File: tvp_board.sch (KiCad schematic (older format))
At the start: 60 parts, among them U1 TVP7002PZP, U4 SN74LVC2G17, U5 AP7361C, U6 TLV70033, U7 NCP703SN19T1G, U9 TLV70019, Y1 ACHL-27MHZ-EK

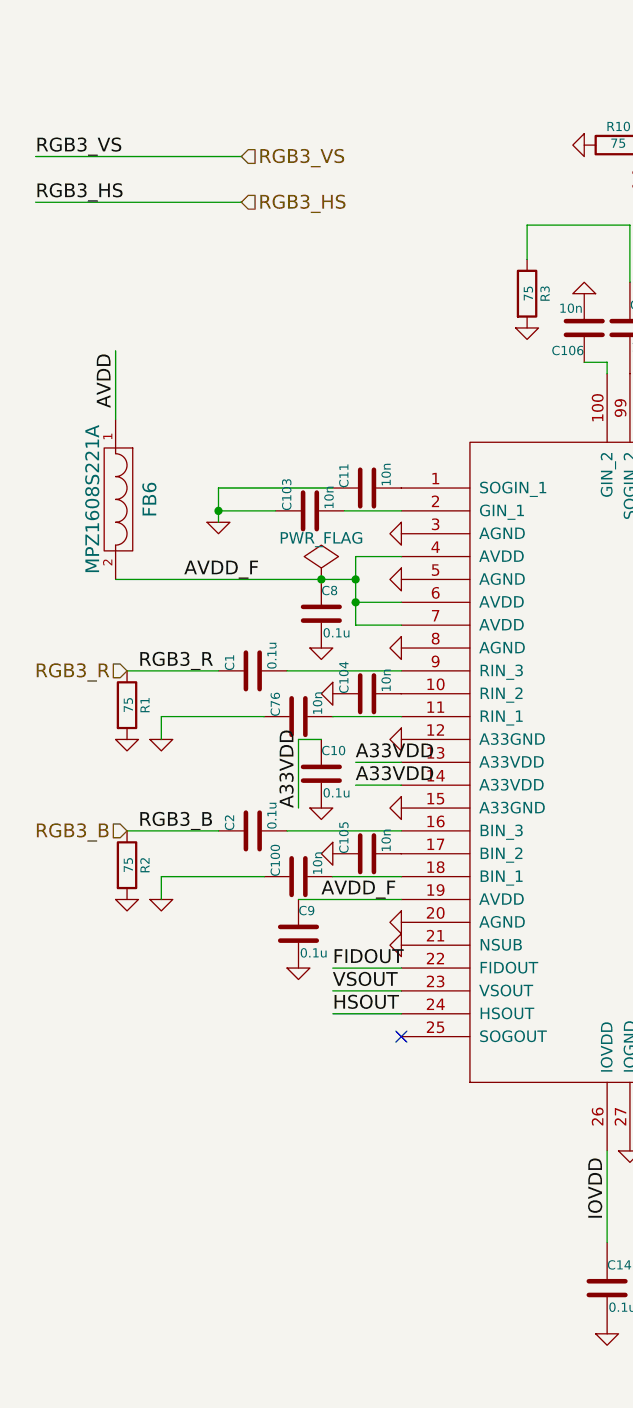
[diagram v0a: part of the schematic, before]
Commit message: update PCB 2
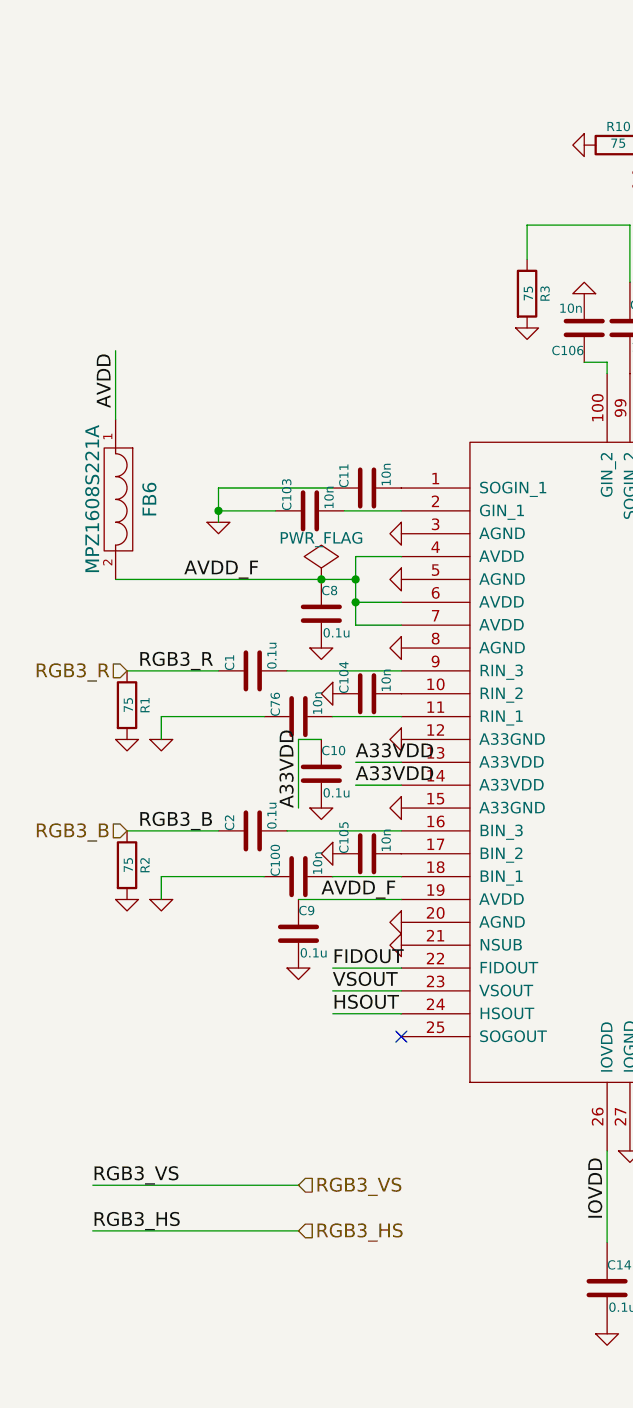
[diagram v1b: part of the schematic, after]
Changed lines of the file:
@@
 Text Label 10950 6550 0    60   ~ 0
 DVDD
-Text Label 2100 1350 0    60   ~ 0
+Text Label 2350 5850 0    60   ~ 0
 RGB3_HS
-Text Label 2100 1150 0    60   ~ 0
+Text Label 2350 5650 0    60   ~ 0
 RGB3_VS
 $Comp
@@
 	7450 6700 7550 6700
 Connection ~ 7450 6950
-Text HLabel 3000 1150 2    60   Input ~ 0
+Text HLabel 3250 5650 2    60   Input ~ 0
 RGB3_VS
-Text HLabel 3000 1350 2    60   Input ~ 0
+Text HLabel 3250 5850 2    60   Input ~ 0
 RGB3_HS
 Wire Wire Line
-	2100 1150 3000 1150
-Wire Wire Line
-	2100 1350 3000 1350
+	2350 5650 3250 5650
+Wire Wire Line
+	2350 5850 3250 5850
 Text HLabel 4800 800  2    60   Input ~ 0
 RGB3_G

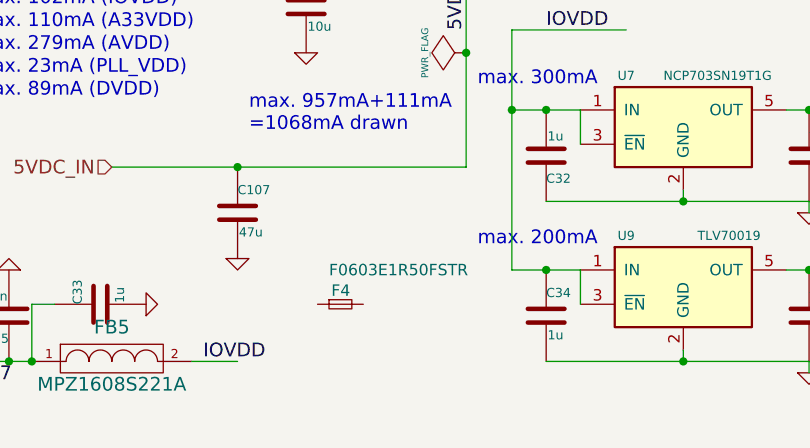
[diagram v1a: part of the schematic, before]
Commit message: update3
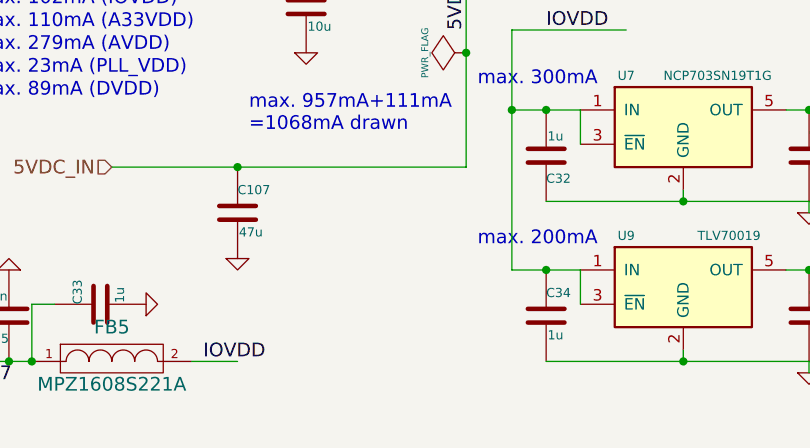
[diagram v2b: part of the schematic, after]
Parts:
- removed F4: F0603E1R50FSTR, Inductor_SMD:L_0603_1608Metric_Pad1.05x0.95mm_HandSolder, symbol ossc_board-rescue:F_Small
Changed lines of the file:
@@
-$EndComp
-$Comp
-L ossc_board-rescue:F_Small F4
-U 1 1 55ECFDAC
-P 8800 6700
-F 0 "F4" H 8760 6760 50  0000 L CNN
-F 1 "F0603E1R50FSTR" H 8750 6850 50  0000 L CNN
-F 2 "Inductor_SMD:L_0603_1608Metric_Pad1.05x0.95mm_HandSolder" H 8800 6700 60  0001 C CNN
-F 3 "" H 8800 6700 60  0000 C CNN
-	1    8800 6700
-	1    0    0    -1
 $EndComp
 $Comp

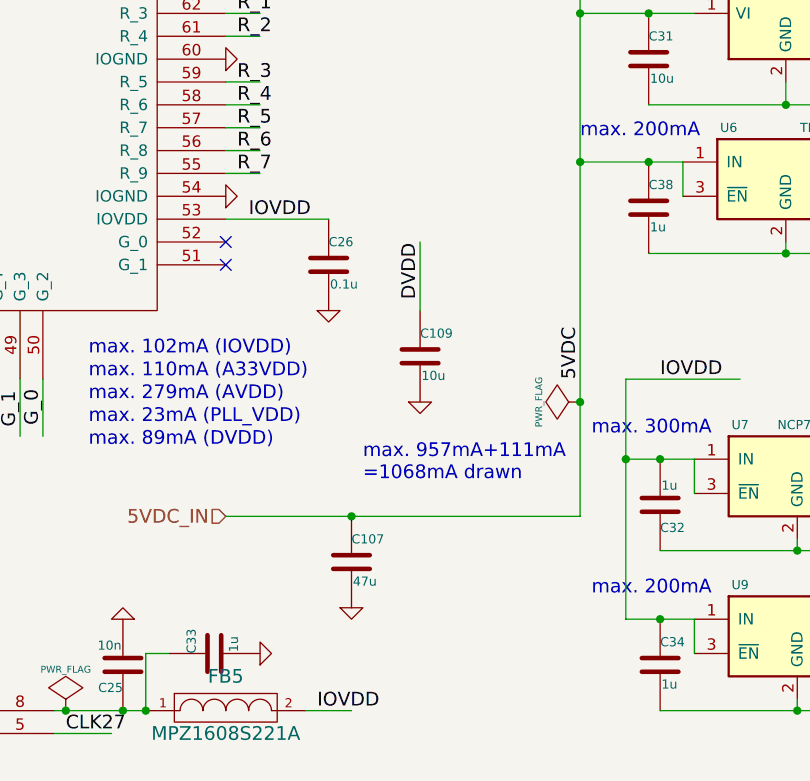
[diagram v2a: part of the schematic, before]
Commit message: minor update
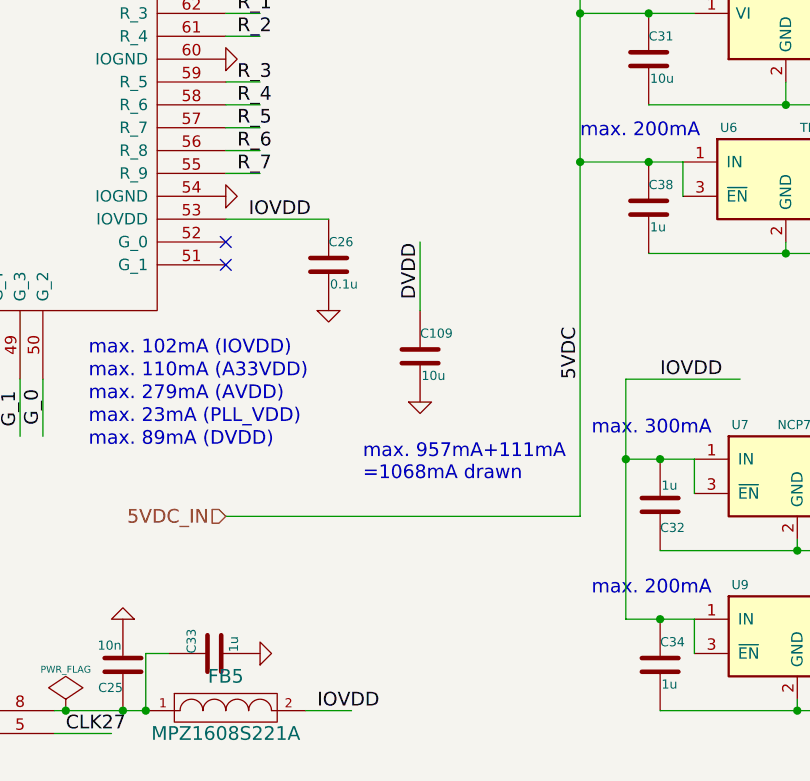
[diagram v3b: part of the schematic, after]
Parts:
- removed C107: 47u, Capacitor_SMD:C_0805_2012Metric_Pad1.15x1.40mm_HandSolder, symbol ossc_board-rescue:C-RESCUE-ossc_board
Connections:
- wire segments 196 -> 194
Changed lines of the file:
@@
 Text Label 9450 2750 0    60   ~ 0
 RESET_N
-$Comp
-L ossc_board-rescue:PWR_FLAG #FLG0131
-U 1 1 54049F52
-P 9350 5600
-F 0 "#FLG0131" H 9350 5695 30  0001 C CNN
-F 1 "PWR_FLAG" H 9350 5780 30  0000 C CNN
-F 2 "" H 9350 5600 60  0001 C CNN
-F 3 "" H 9350 5600 60  0000 C CNN
-	1    9350 5600
-	0    -1   -1   0
-$EndComp
 NoConn ~ 5700 5500
 NoConn ~ 5800 5500
@@
 $EndComp
 $Comp
-L ossc_board-rescue:C-RESCUE-ossc_board C107
-U 1 1 55EC52FF
-P 8350 6300
-F 0 "C107" H 8350 6400 40  0000 L CNN
-F 1 "47u" H 8356 6215 40  0000 L CNN
-F 2 "Capacitor_SMD:C_0805_2012Metric_Pad1.15x1.40mm_HandSolder" H 8388 6150 30  0001 C CNN
-F 3 "~" H 8350 6300 60  0000 C CNN
-	1    8350 6300
-	1    0    0    -1
-$EndComp
-$Comp
-L ossc_board-rescue:GND-RESCUE-ossc_board #PWR0150
-U 1 1 55EC5BFD
-P 8350 6500
-F 0 "#PWR0150" H 8350 6500 30  0001 C CNN
-F 1 "GND" H 8350 6430 30  0001 C CNN
-F 2 "" H 8350 6500 60  0001 C CNN
-F 3 "" H 8350 6500 60  0000 C CNN
-	1    8350 6500
-	1    0    0    -1
-$EndComp
-$Comp
 L ossc_board-rescue:FILTER FB6
 U 1 1 55F21890
@@
 	8350 6950 8150 6950
 Connection ~ 7100 6950
-Connection ~ 9350 5600
 Wire Wire Line
 	9450 3200 9900 3200
@@
 	10250 4300 10800 4300
 Wire Wire Line
-	9350 4550 9350 5600
-Wire Wire Line
 	9350 3900 9350 4550
 Wire Wire Line
@@
 Wire Wire Line
 	7100 6950 7350 6950
-Wire Wire Line
-	9350 5600 9350 6100
 Wire Wire Line
 	9550 5850 9550 6550
@@
 Text HLabel 2500 4100 0    60   Input ~ 0
 RGB3_B
-Wire Wire Line
-	9350 6100 8350 6100
-Connection ~ 8350 6100
 Text HLabel 7800 6100 0    60   Input ~ 0
 5VDC_IN
 Wire Wire Line
-	7800 6100 8350 6100
+	7800 6100 9350 6100
+Wire Wire Line
+	9350 4550 9350 6100
 $EndSCHEMATC
